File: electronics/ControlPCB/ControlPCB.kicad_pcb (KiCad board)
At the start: 2 copper layers, 99.8 x 67.4 mm, 70 parts, among them P1 CONN_02X03, P2 CONN_02X03, P3 CONN_02X03, P4 CONN_02X03, P5 CONN_02X03, P6 CONN_02X03, P7 CONN_02X03, P8 CONN_02X03, U1 POLOLU_A4988, U2 POLOLU_A4988, U3 POLOLU_A4988, U4 POLOLU_A4988, U5 POLOLU_A4988, U6 POLOLU_A4988, U7 POLOLU_A4988, U8 POLOLU_A4988

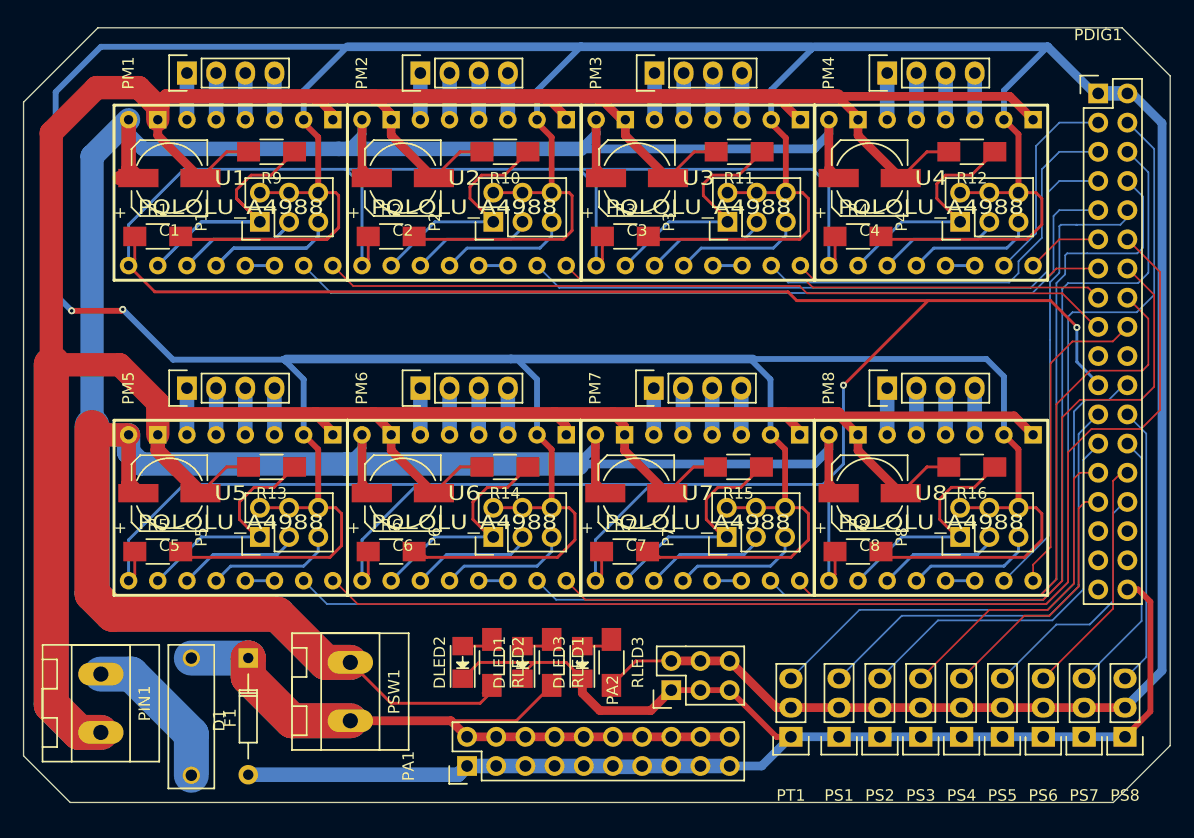
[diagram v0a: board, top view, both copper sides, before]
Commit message: mistakes were made
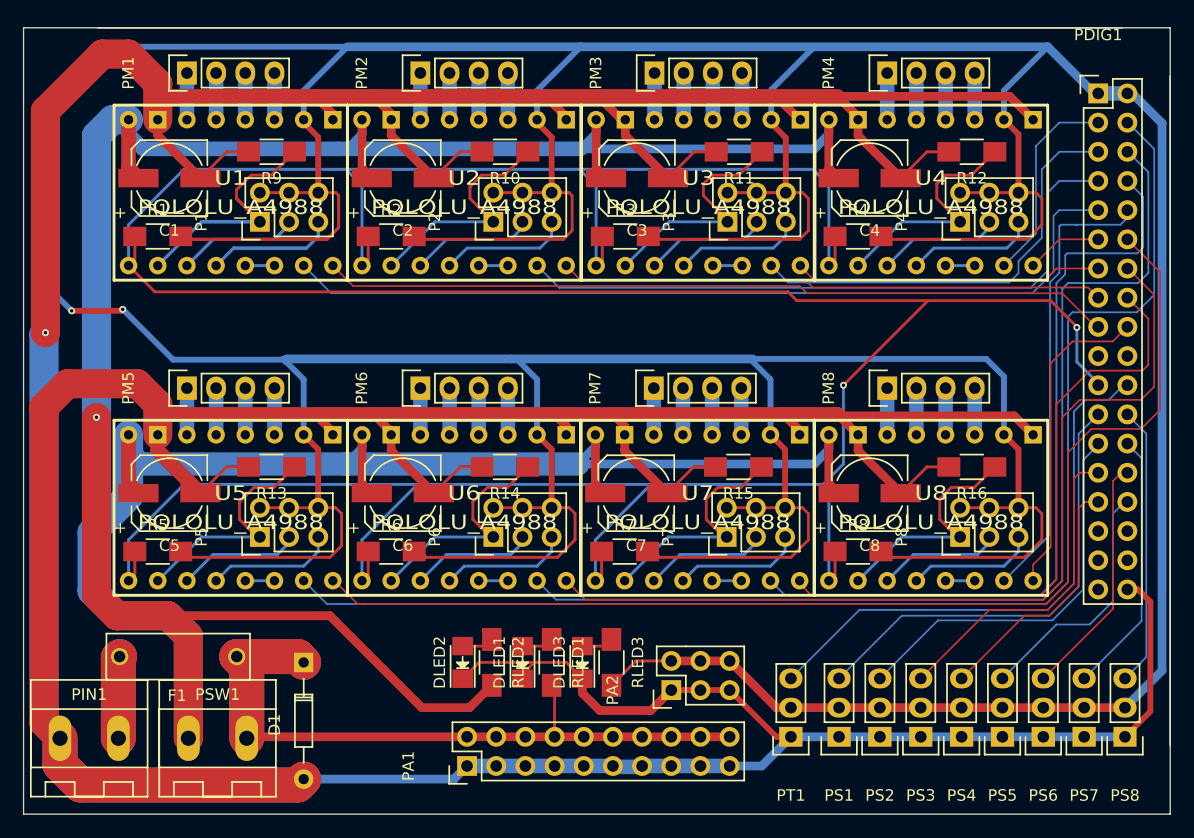
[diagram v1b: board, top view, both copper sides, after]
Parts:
- moved PSW1 9.14 mm to (110.9, 133.9), turned to 180 degrees
- moved F1 5.36 mm to (104.9, 126.7), turned to 180 degrees
- moved D1 4.84 mm to (115.8, 127.3)
- moved PIN1 1.61 mm to (99.7, 133.9), turned to 180 degrees
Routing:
- net GND: track 528.0 -> 570.7 mm, vias 0 -> 1
- net +12V: track 321.5 -> 319.9 mm, vias 0 -> 1
- net VDD: track 73.7 -> 74.5 mm
- net Net-(F1-Pad2): track 13.6 -> 14.3 mm
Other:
- board size 99.8 x 67.4 mm -> 99.8 x 68.5 mm
